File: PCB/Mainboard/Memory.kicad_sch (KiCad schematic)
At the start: 29 parts, among them J15 RAM Module, U28 M5M4V16160BTP, U33 M5M4V16160BTP

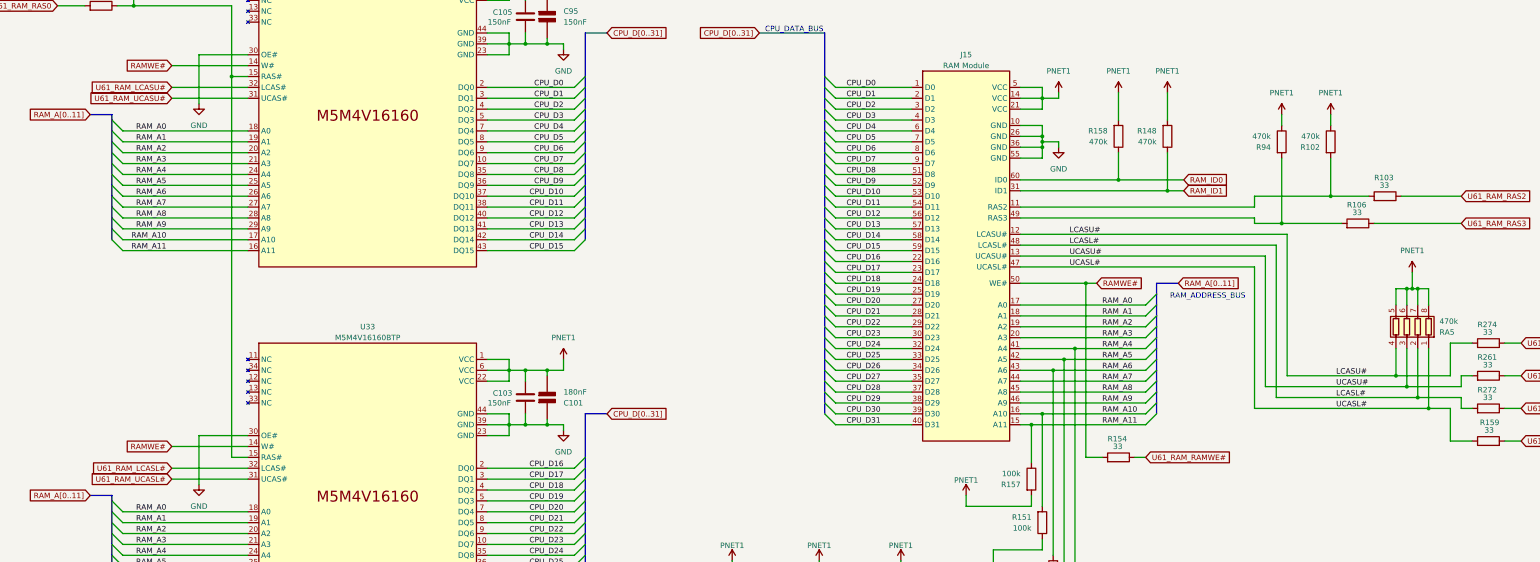
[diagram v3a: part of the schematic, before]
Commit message: Add files via upload
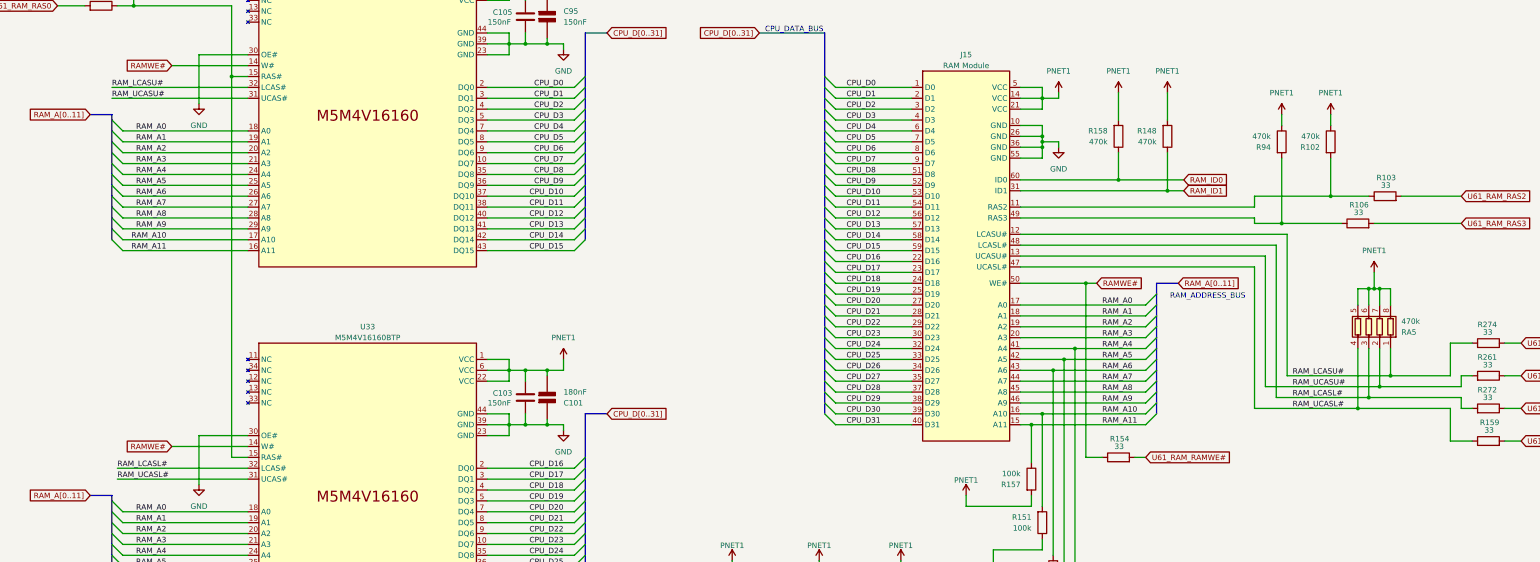
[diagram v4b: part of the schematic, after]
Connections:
- net RAMWE#: now also R154.1; no longer R154.2
- net U61_RAM_LCASL#: no longer U33.32 (LCAS#)
- net U61_RAM_LCASU#: no longer U28.32 (LCAS#)
- net U61_RAM_RAMWE#: now also R154.2; no longer R154.1
- net U61_RAM_RAS2: now also R103.2; no longer R103.1
- net U61_RAM_RAS3: now also R106.2; no longer R106.1
- net U61_RAM_UCASL#: no longer U33.31 (UCAS#)
- net U61_RAM_UCASU#: no longer U28.31 (UCAS#)
- net at J15.11 (RAS2), R102.2: now also R103.1; no longer R103.2
- net at J15.49 (RAS3), R94.2: now also R106.1; no longer R106.2
- net LCASL# renamed RAM_LCASL#
- net RAM_LCASL#: now also RA5.3 (R3.1), U33.32 (LCAS#); no longer RA5.2 (R2.1)
- net LCASU# renamed RAM_LCASU#
- net RAM_LCASU#: now also RA5.1 (R1.1), U28.32 (LCAS#); no longer RA5.4 (R4.1)
- net UCASL# renamed RAM_UCASL#
- net RAM_UCASL#: now also RA5.4 (R4.1), U33.31 (UCAS#); no longer RA5.1 (R1.1)
- net UCASU# renamed RAM_UCASU#
- net RAM_UCASU#: now also RA5.2 (R2.1), U28.31 (UCAS#); no longer RA5.3 (R3.1)
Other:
- moved on the sheet: R103, R106, R154, RA5
